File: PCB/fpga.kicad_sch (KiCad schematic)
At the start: 40 parts, among them IC1 S25FL256LAGMFI003, U4 XC7A100T-FTG256, Y2 ECS-3953M-400-BN-TR

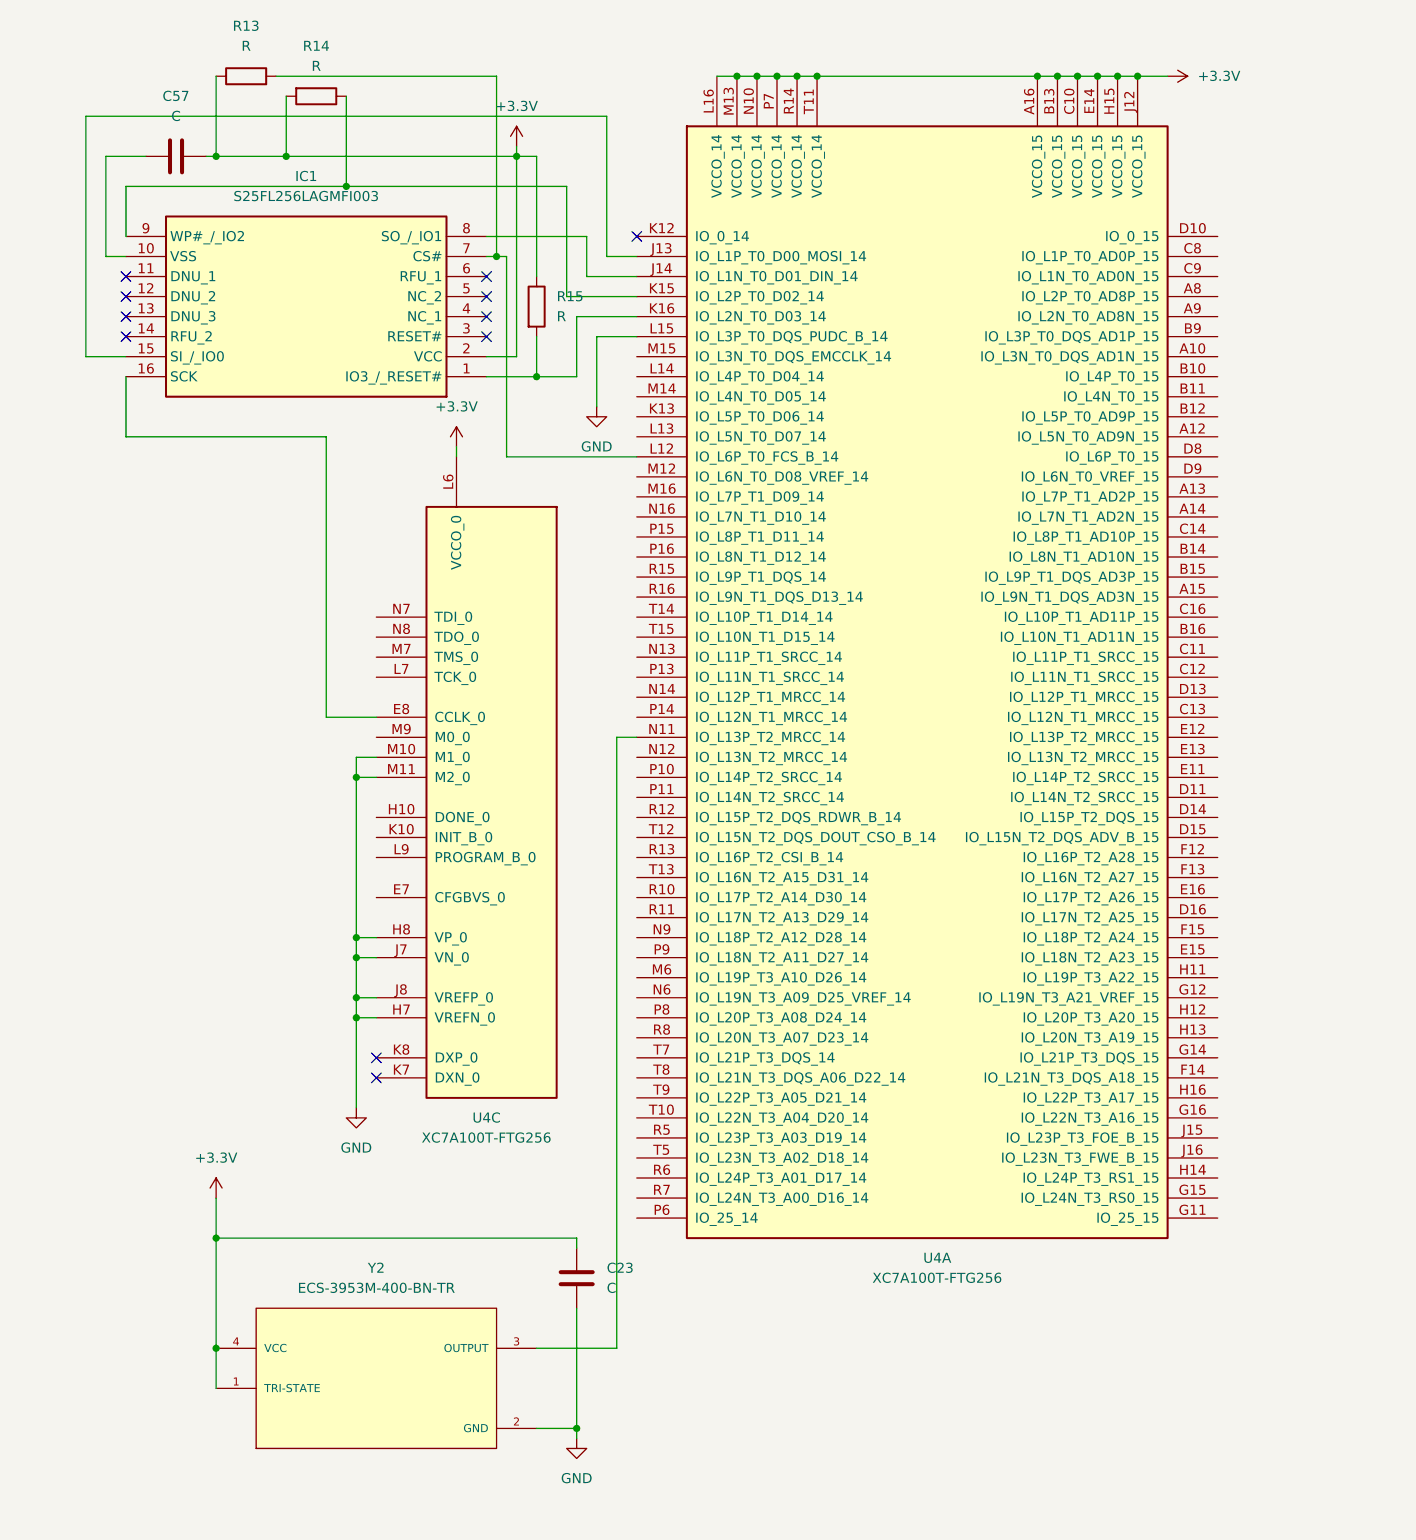
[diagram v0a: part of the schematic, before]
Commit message: Debugg added, missing one unit still
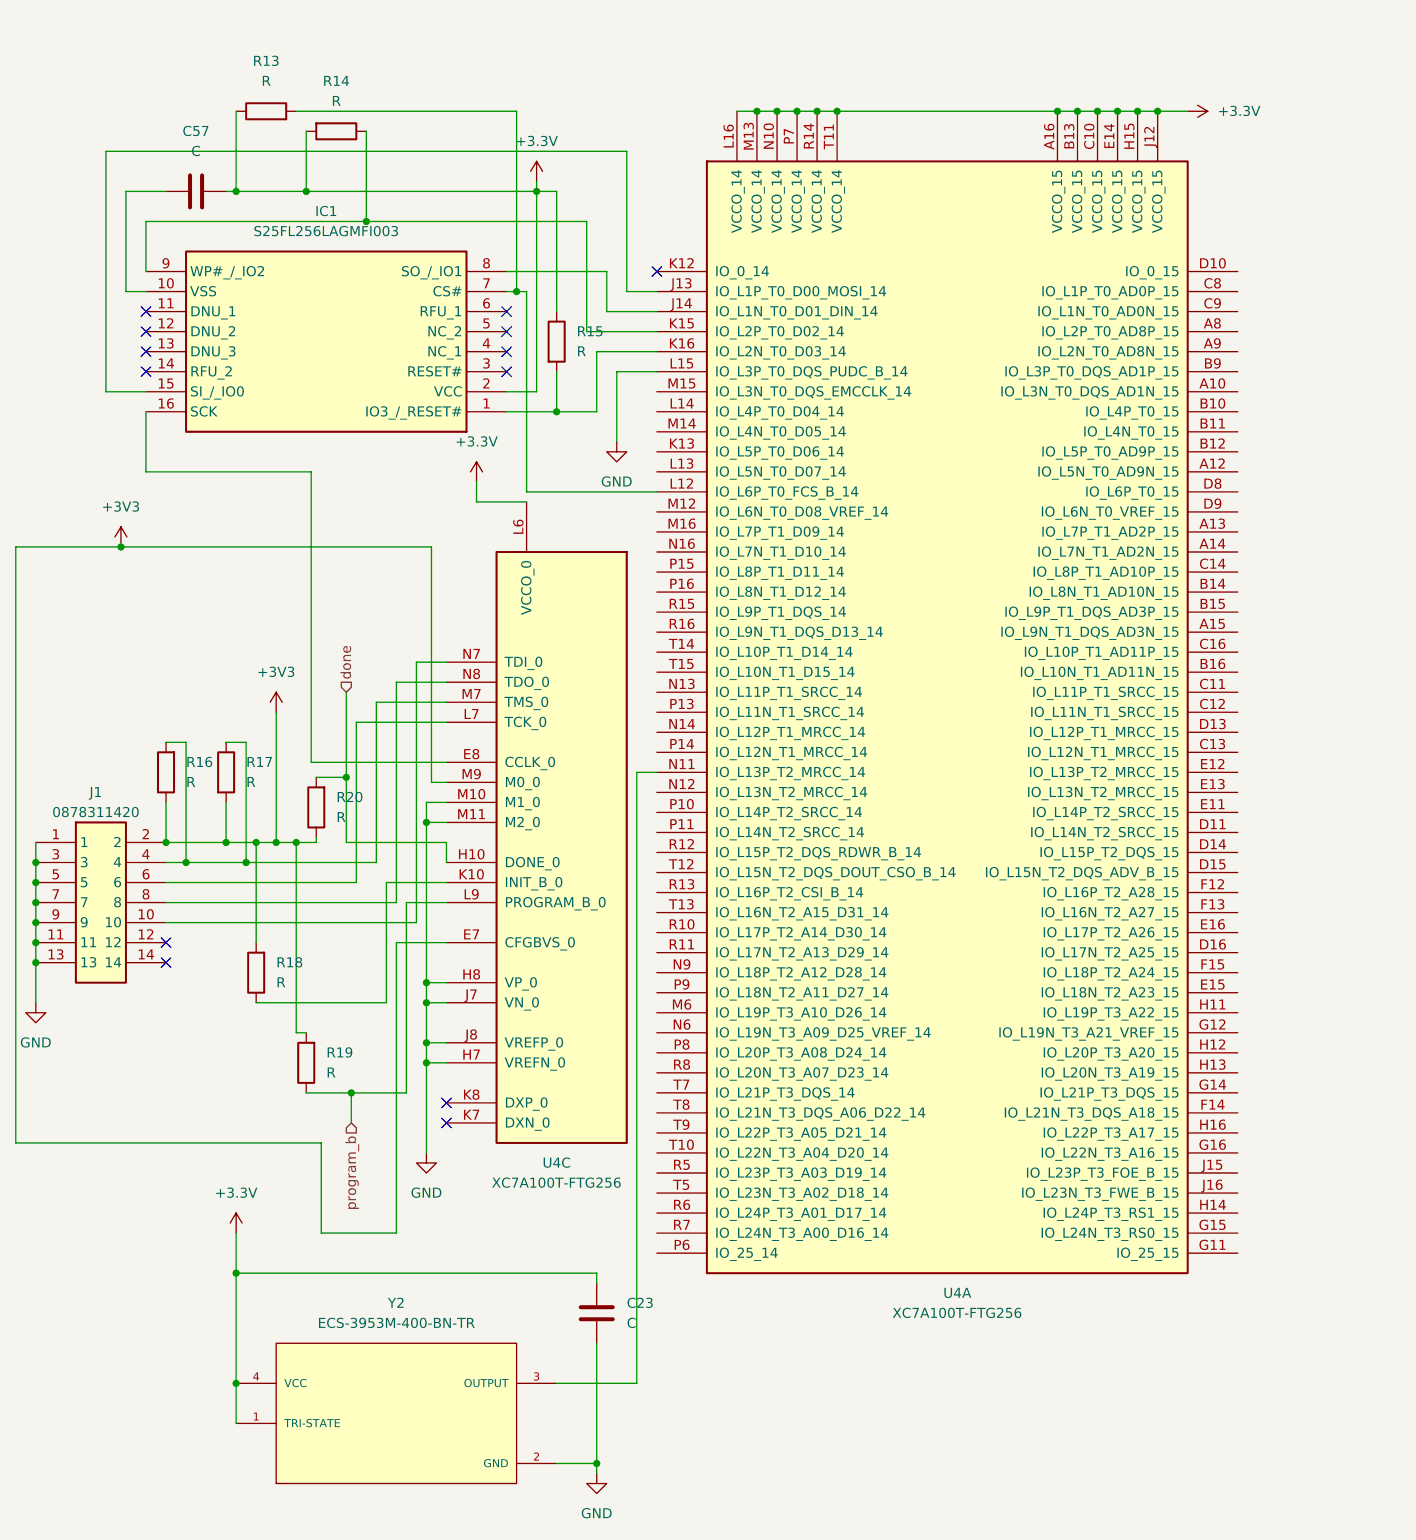
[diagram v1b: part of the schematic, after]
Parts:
- added J1: 0878311420, 0878311420, symbol 0878311420:0878311420
- added R16, R17, R18, R19, R20: R, symbol Device:R
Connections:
- net GND: now also J1.1, J1.11, J1.13, J1.3, J1.5, J1.7, J1.9
- net +3V3: now reaches U4.E7 (CFGBVS_0)
- net +3V3: now also U4.M9 (M0_0), J1.2, R16.1, R17.2, R18.2, R19.2, R20.1
- net done: now reaches U4.H10 (DONE_0)
- net done: now also R20.2
- net at U4.K10 (INIT_B_0): now also R18.1
- net at U4.L7 (TCK_0): now also J1.6
- net program_b: now reaches U4.L9 (PROGRAM_B_0)
- net program_b: now also R19.1
- net at U4.M7 (TMS_0): now also J1.4, R16.2, R17.1
- net at U4.N7 (TDI_0): now also J1.10
- net at U4.N8 (TDO_0): now also J1.8
- no-connect marks 11 -> 13
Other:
- moved on the sheet: C23, C57, IC1, R13, R14, R15, U4A, U4C, Y2

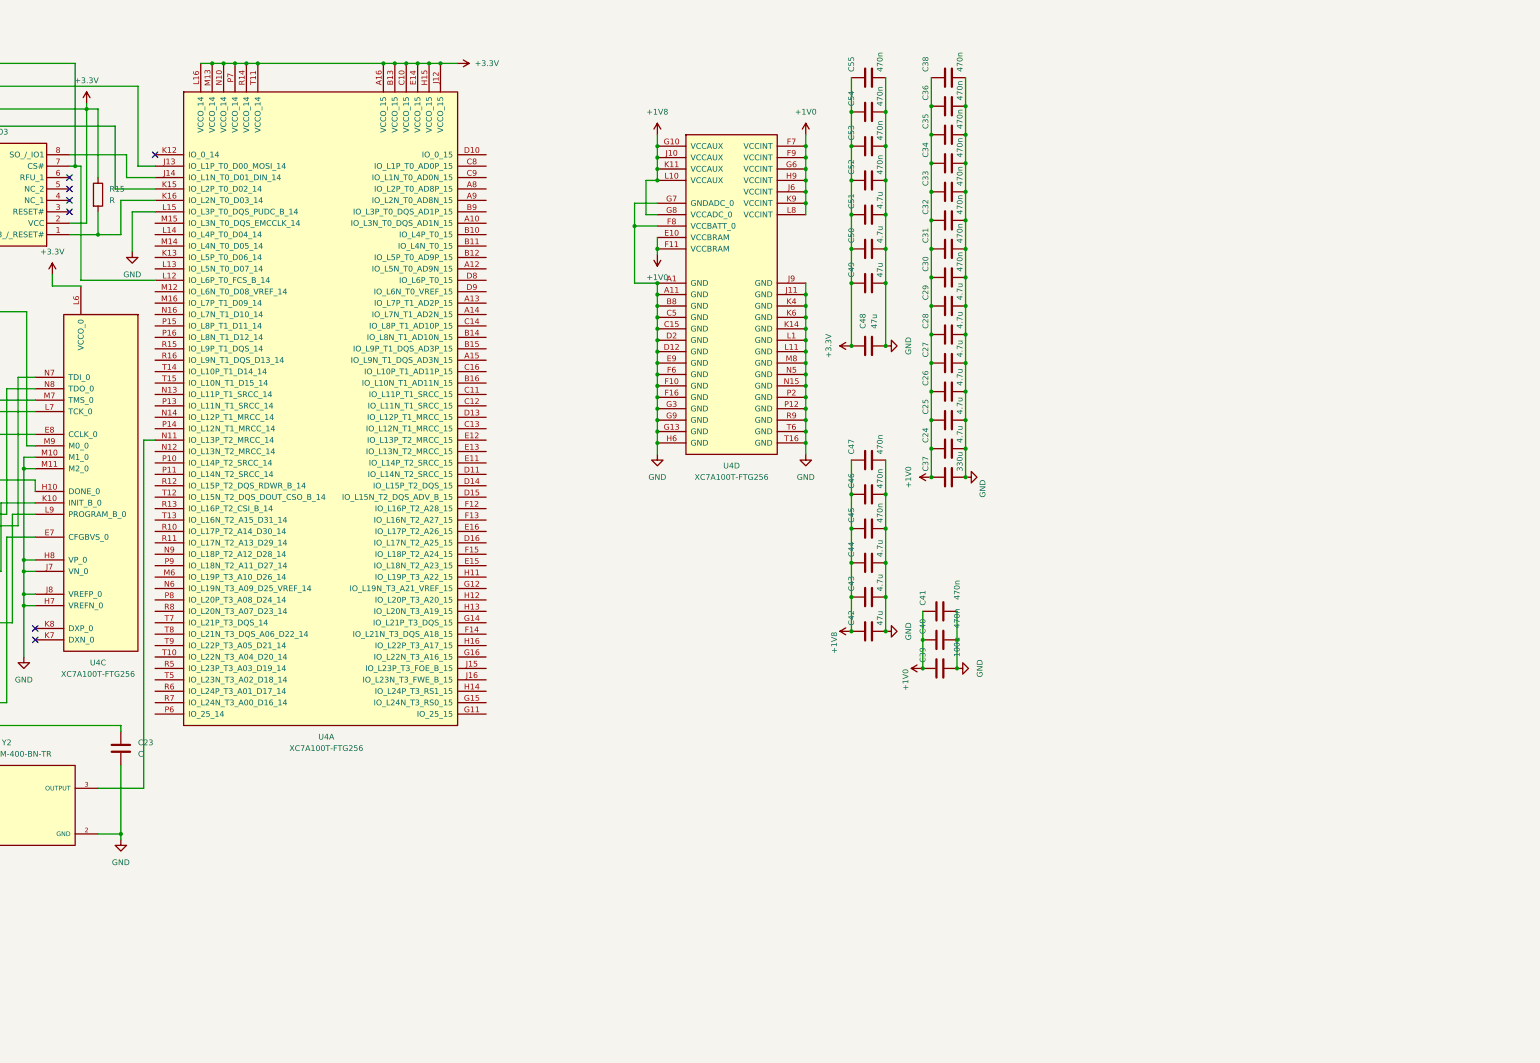
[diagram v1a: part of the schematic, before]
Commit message: Work
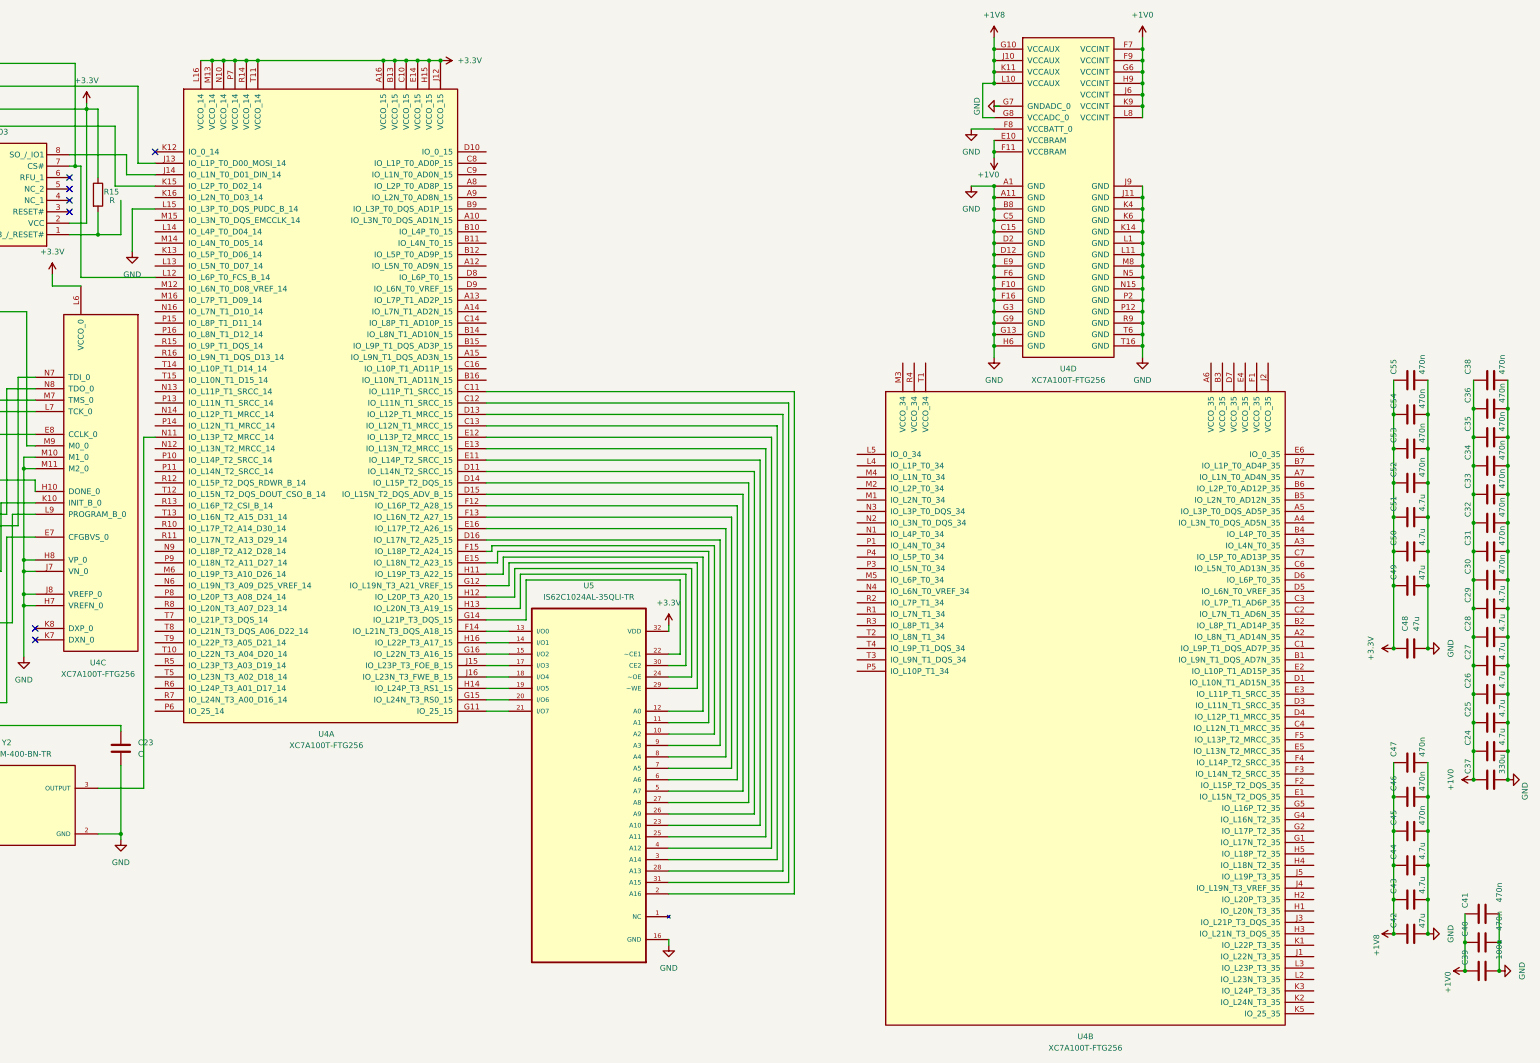
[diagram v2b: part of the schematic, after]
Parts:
- added unit 2 of U4
- added U5: IS62C1024AL-35QLI-TR, IS62C1024AL-35QLI-TR:SOIC127P1412X305-32N, symbol IS62C1024AL-35QLI-TR:IS62C1024AL-35QLI-TR
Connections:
- net +3.3V: now also U5.32 (VDD)
- net GND: now also U5.16 (GND)
- net at U4.C11 (IO_L11P_T1_SRCC_15): now also U5.2 (A16)
- net at U4.C12 (IO_L11N_T1_SRCC_15): now also U5.31 (A15)
- net at U4.C13 (IO_L12N_T1_MRCC_15): now also U5.3 (A14)
- net at U4.D11 (IO_L14N_T2_SRCC_15): now also U5.26 (A9)
- net at U4.D13 (IO_L12P_T1_MRCC_15): now also U5.28 (A13)
- net at U4.D14 (IO_L15P_T2_DQS_15): now also U5.27 (A8)
- net at U4.D15 (IO_L15N_T2_DQS_ADV_B_15): now also U5.5 (A7)
- net at U4.D16 (IO_L17N_T2_A25_15): now also U5.9 (A3)
- net at U4.E11 (IO_L14P_T2_SRCC_15): now also U5.23 (A10)
- net at U4.E12 (IO_L13P_T2_MRCC_15): now also U5.4 (A12)
- net at U4.E13 (IO_L13N_T2_MRCC_15): now also U5.25 (A11)
- net at U4.E15 (IO_L18N_T2_A23_15): now also U5.11 (A1)
- net at U4.E16 (IO_L17P_T2_A26_15): now also U5.8 (A4)
- net at U4.F12 (IO_L16P_T2_A28_15): now also U5.6 (A6)
- net at U4.F13 (IO_L16N_T2_A27_15): now also U5.7 (A5)
- net at U4.F14 (IO_L21N_T3_DQS_A18_15): now also U5.13 (I/O0)
- net at U4.F15 (IO_L18P_T2_A24_15): now also U5.10 (A2)
- net at U4.G11 (IO_25_15): now also U5.21 (I/O7)
- net at U4.G12 (IO_L19N_T3_A21_VREF_15): now also U5.29 (~WE)
- net at U4.G14 (IO_L21P_T3_DQS_15): now also U5.22 (~CE1)
- net at U4.G15 (IO_L24N_T3_RS0_15): now also U5.20 (I/O6)
- net at U4.G16 (IO_L22N_T3_A16_15): now also U5.15 (I/O2)
- net at U4.H11 (IO_L19P_T3_A22_15): now also U5.12 (A0)
- net at U4.H12 (IO_L20P_T3_A20_15): now also U5.24 (~OE)
- net at U4.H13 (IO_L20N_T3_A19_15): now also U5.30 (CE2)
- net at U4.H14 (IO_L24P_T3_RS1_15): now also U5.19 (I/O5)
- net at U4.H16 (IO_L22P_T3_A17_15): now also U5.14 (I/O1)
- net at U4.J15 (IO_L23P_T3_FOE_B_15): now also U5.17 (I/O3)
- net at U4.J16 (IO_L23N_T3_FWE_B_15): now also U5.18 (I/O4)
- net at IC1.1 (IO3_/_RESET#), R15.2: no longer U4.K16 (IO_L2N_T0_D03_14)
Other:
- moved on the sheet: C24, C25, C26, C27, C28, C29, C30, C31, C32, C33, C34, C35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
